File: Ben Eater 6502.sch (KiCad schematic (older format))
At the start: 5 parts, among them SW1 Reset, U1 W65C02SxP, U2 4011, U3 28C256

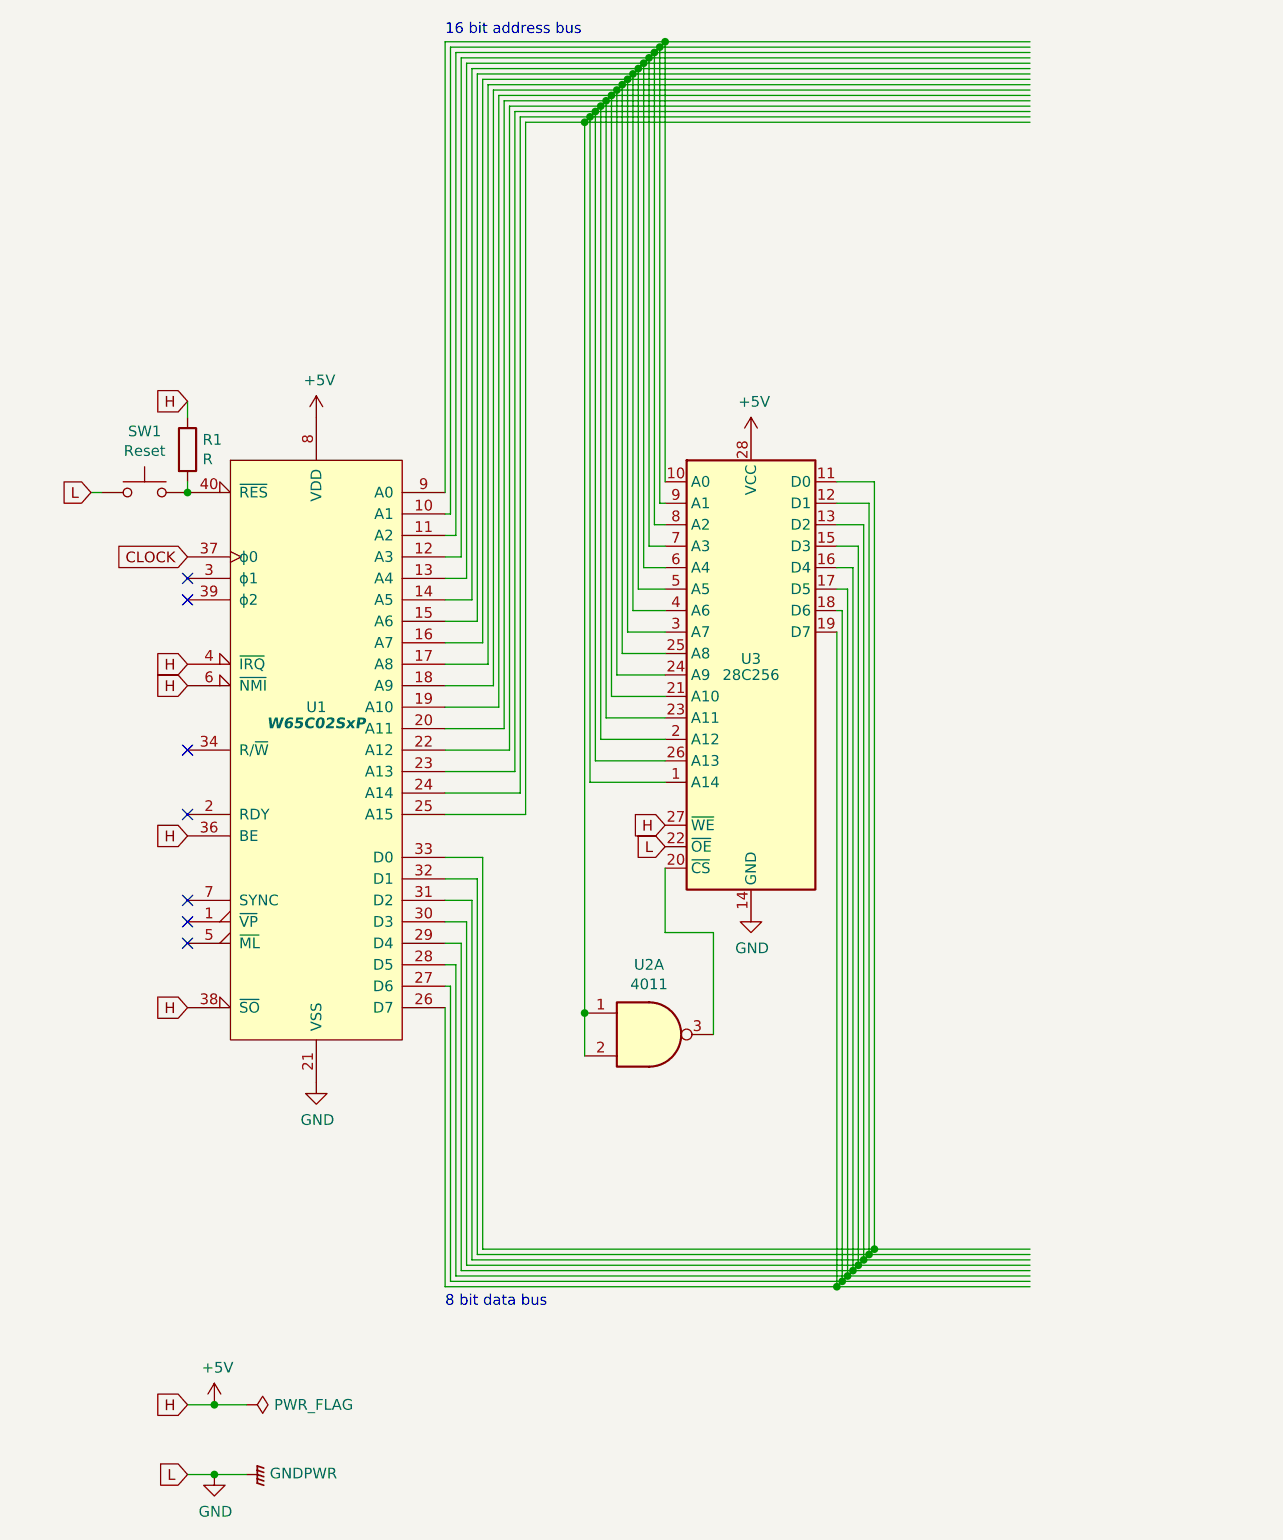
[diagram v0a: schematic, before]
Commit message: Stage 2b
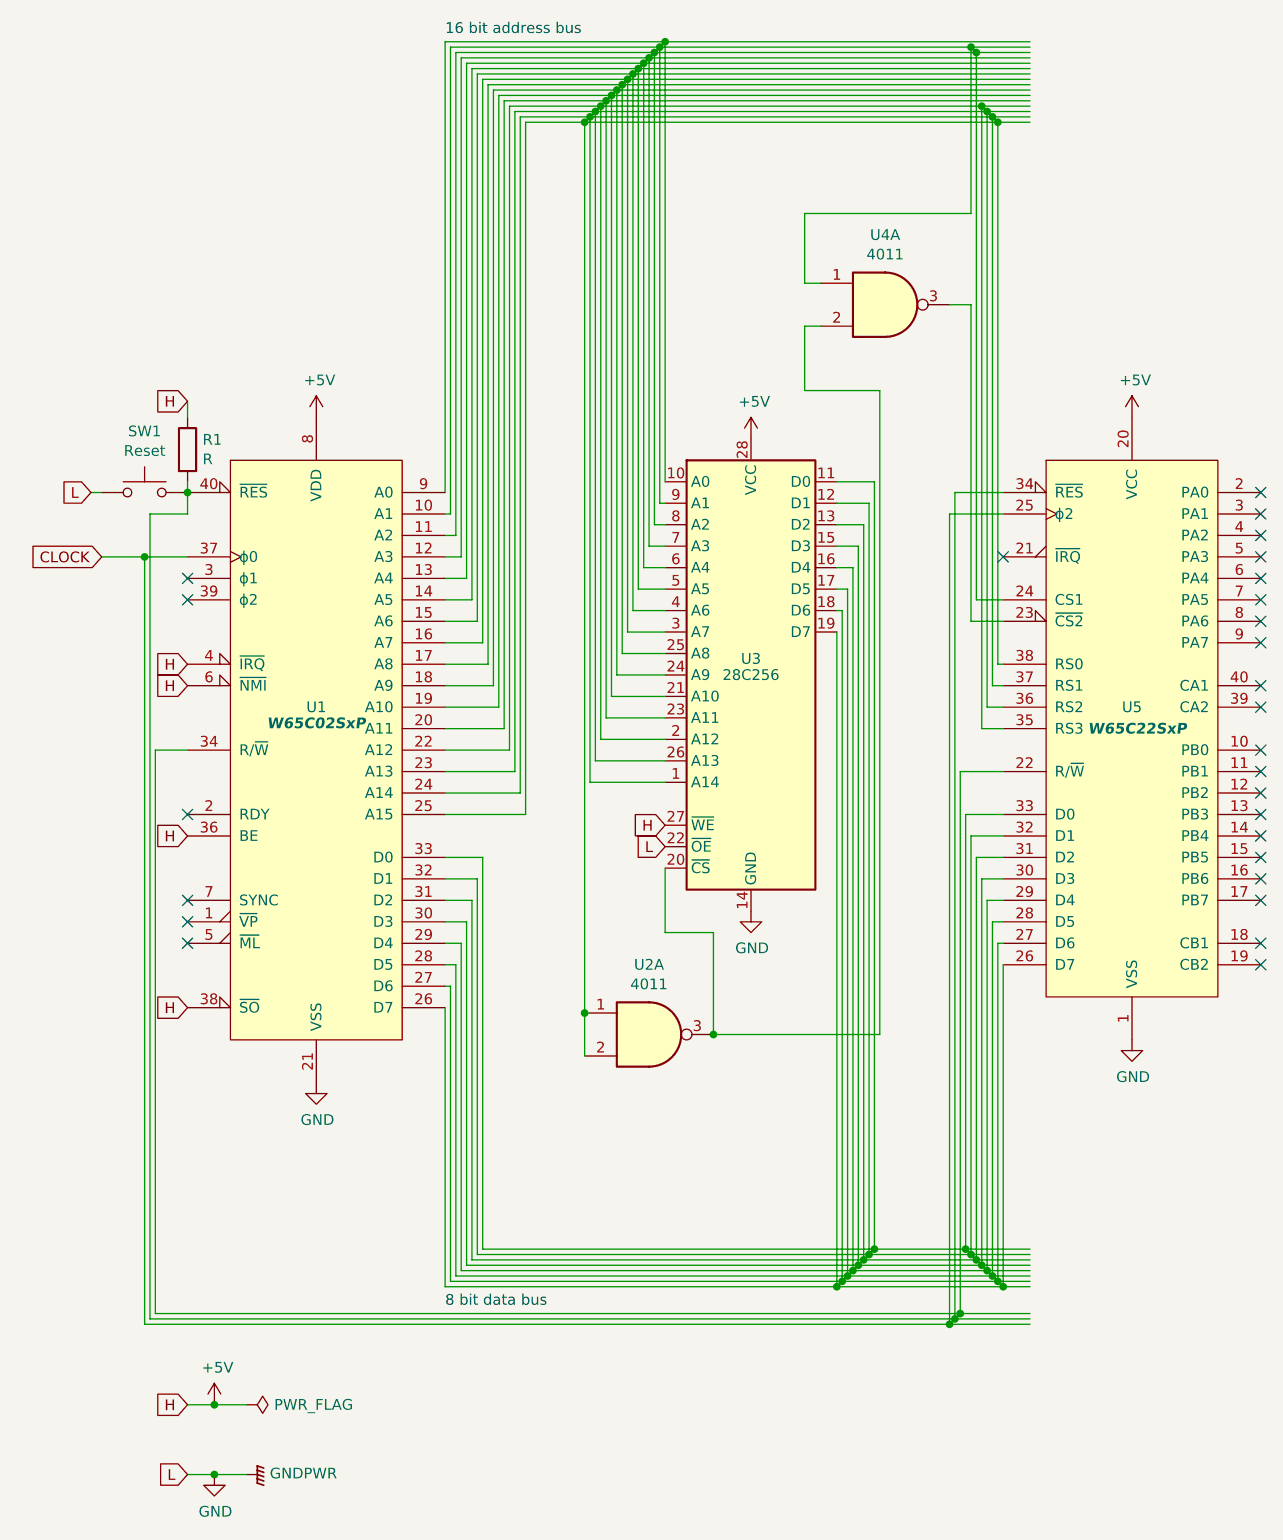
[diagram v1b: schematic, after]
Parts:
- added U4: 4011, symbol 4xxx:4011
- added U5: W65C22SxP, symbol 65xx:W65C22SxP
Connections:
- wire segments 150 -> 221
- no-connect marks 7 -> 27
